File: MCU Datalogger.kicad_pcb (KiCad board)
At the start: 2 copper layers, 50 x 33.4 mm, 30 parts, among them J1 Conn_01x04_Pin, J2 Conn_01x09_Pin, J3 Conn_01x04_Pin, J4 Conn_02x03_Odd_Even, U1 24LC1025, U2 24LC1025, U3 DS1337S_, U4 ATMEGA328P-AU, Y1 32.768 KHz, Y2 16 MHz

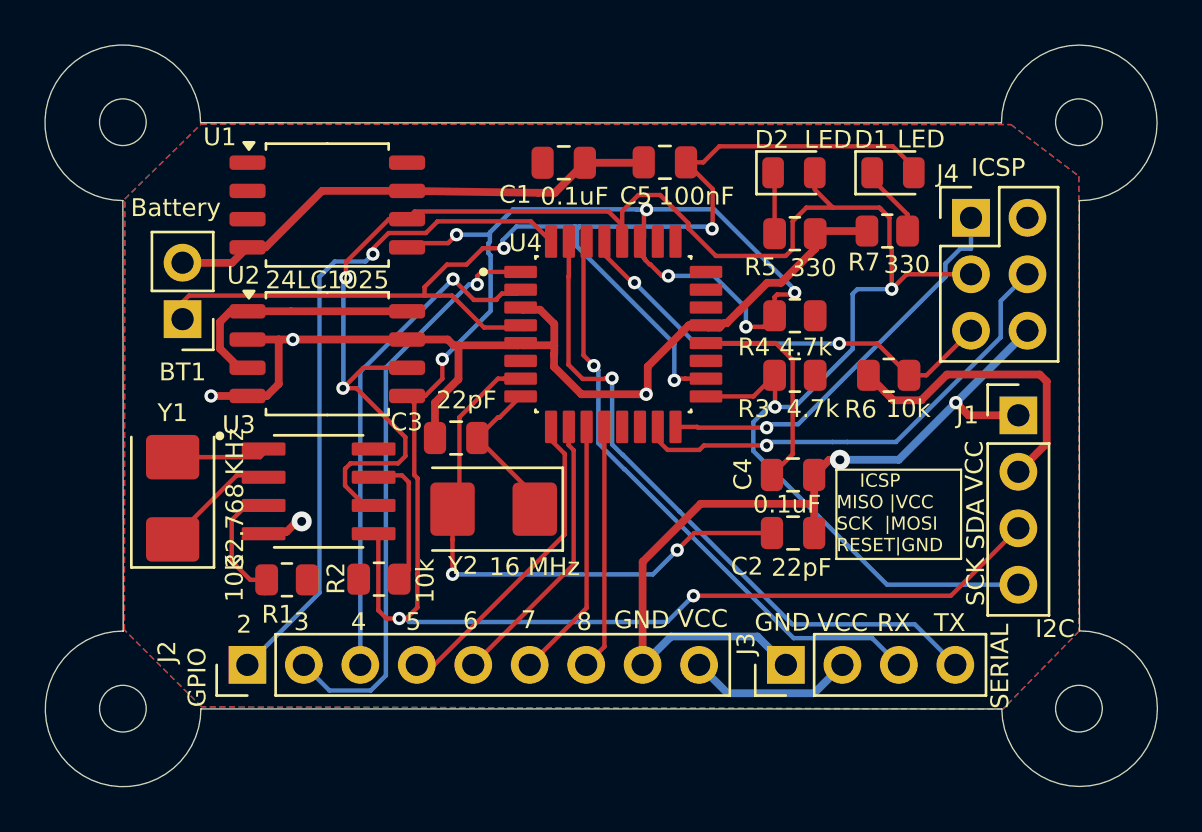
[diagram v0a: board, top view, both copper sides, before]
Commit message: added the gerber files.
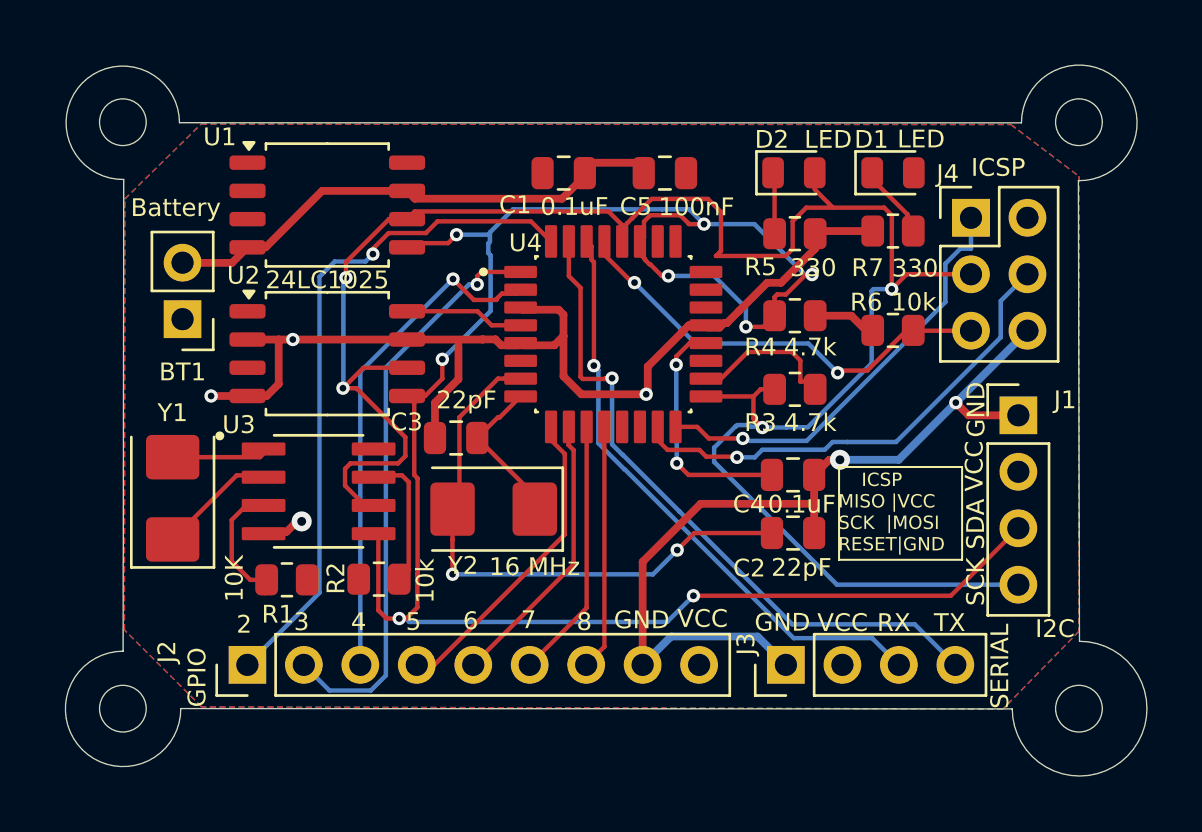
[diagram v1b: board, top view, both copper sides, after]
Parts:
- moved R6 2.03 mm to (144.9, 92.7)
- moved R3 0.63 mm to (140.5, 95.3)
- moved C5 0.48 mm to (134.7, 85.6)
- moved C1 0.47 mm to (130.1, 85.6)
- moved R7 0.26 mm to (144.9, 88.2)
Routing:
- net /Vcc: track 91.2 -> 17.5 mm, vias 3 -> 0
- net /SCK: track 91.2 -> 95.7 mm
- net /SDA: track 87.2 -> 90.8 mm
- net GND: track 110.7 -> 112.4 mm
- net Net-(U4-AREF): track 9.77 -> 11.1 mm, vias 0 -> 2
- net /MISO: track 18.4 -> 19.5 mm
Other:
- board size 50 x 33.4 mm -> 48.6 x 32 mm
